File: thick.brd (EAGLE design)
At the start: 37 x 25 mm, 27 parts, among them J1 43045-0400, J4 F1003WR-S-06PT, Q1 SI2319DDS-T1-GE3, U1 ATTINY85-20SU

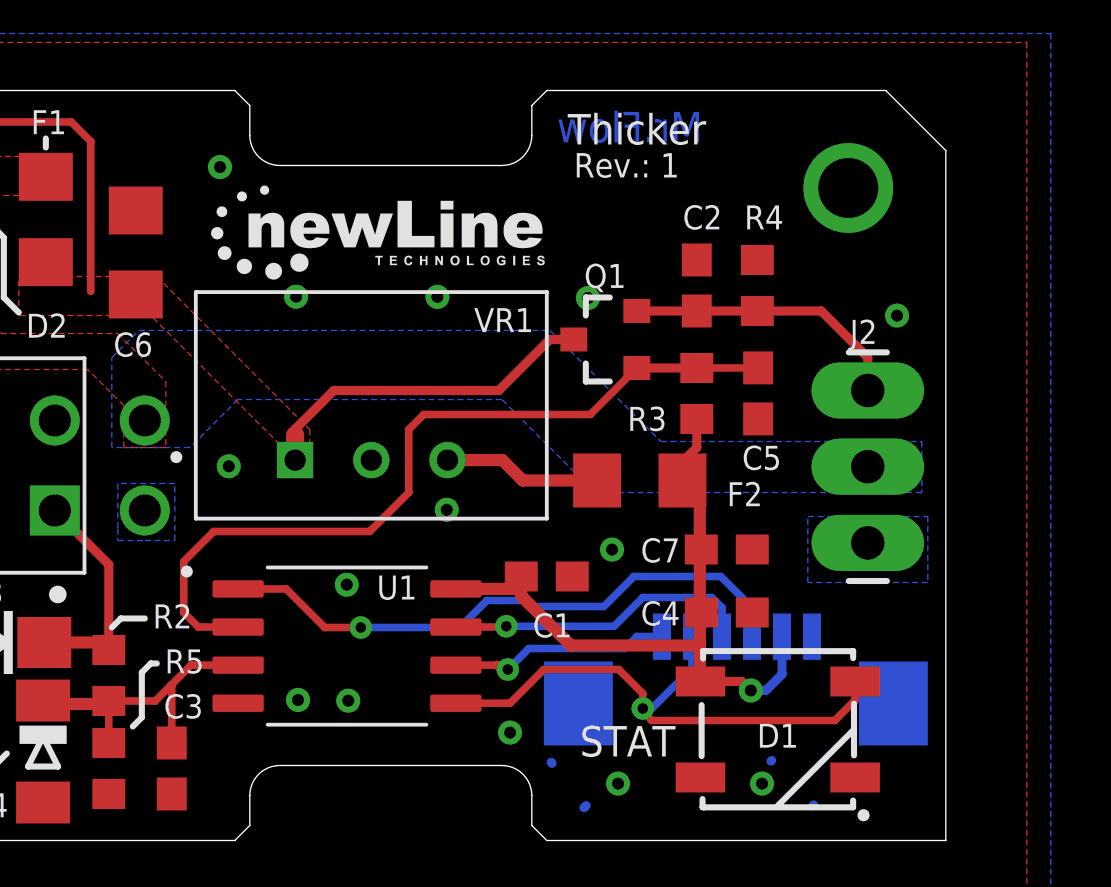
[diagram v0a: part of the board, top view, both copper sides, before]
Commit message: Javított végleges
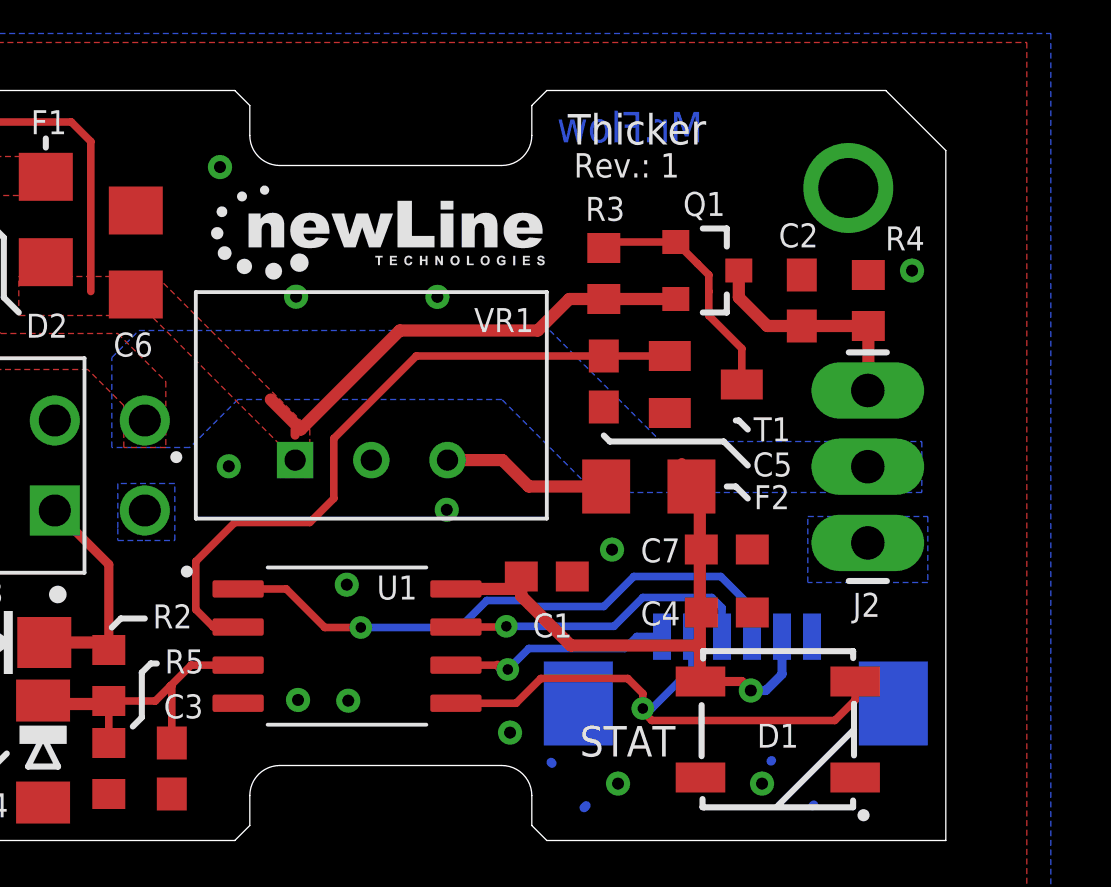
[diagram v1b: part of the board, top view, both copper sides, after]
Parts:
- added T1: (no value), transistor:SC59-BEC
- moved C5 5.16 mm to (25.6, 15.3)
- moved R3 5.06 mm to (25.6, 18.9)
- moved Q1 4.02 mm to (29.0, 19.0), turned to 270 degrees
- moved R4 3.73 mm to (34.4, 18.0)
- moved C2 3.54 mm to (32.2, 18.0)
- moved F2 0.36 mm to (27.1, 11.8)
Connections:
- removed net !IGN_EN: C5.1, Q1.1, R3.1, U1.2
- new net IGN_EN: C5.1, T1.B, U1.2
- new net N$1: Q1.1, R3.1, T1.C
- net 5V: no longer R3.2
- net GND: now also T1.E
- net IGNITION: now also Q1.3; no longer Q1.2
- net VDD: now also Q1.2, R3.2; no longer Q1.3
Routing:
- net !IGN_EN: track 26.8 -> 0.00 mm
- net IGN_EN: track 0.00 -> 23.1 mm
- net N$1: track 0.00 -> 8.14 mm
- net VDD: track 24.0 -> 28.2 mm
- net IGNITION: track 9.44 -> 7.77 mm
- net 5V: track 23.6 -> 22.0 mm
- net GND: vias 19 -> 18

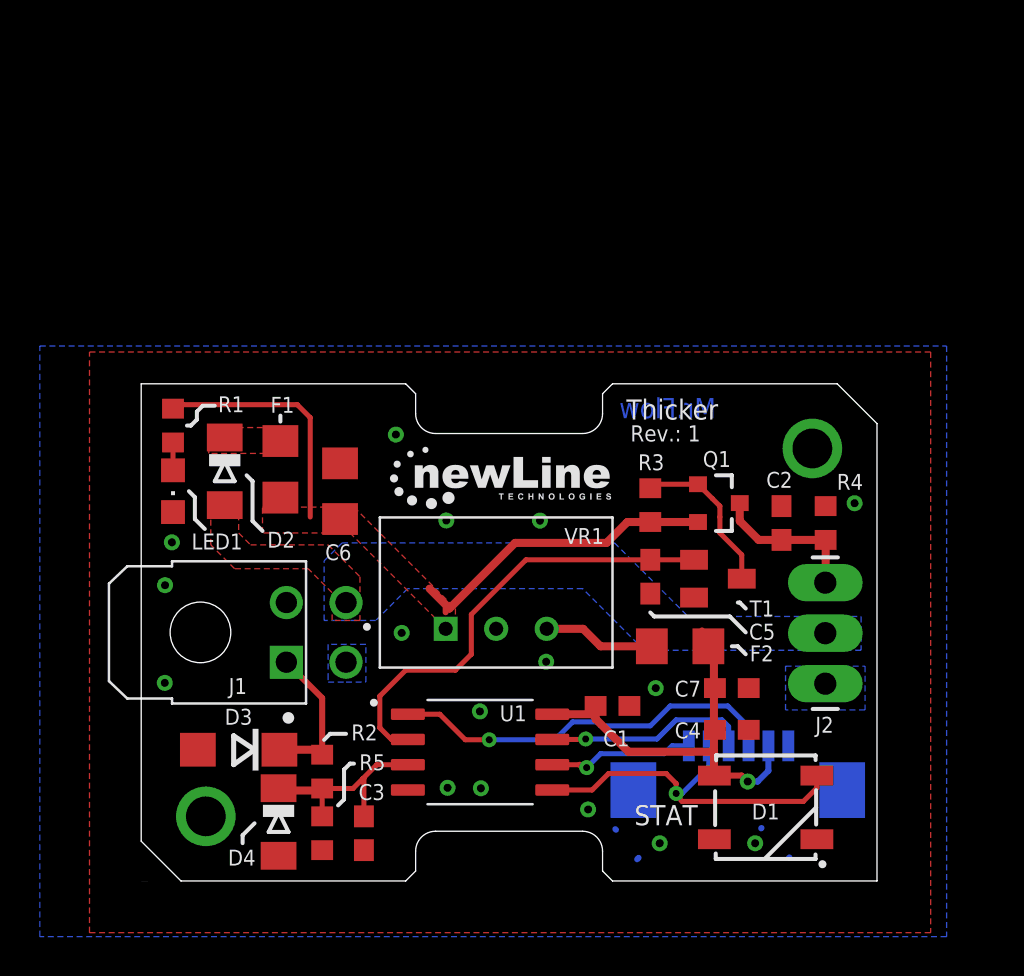
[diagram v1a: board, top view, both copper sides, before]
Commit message: rev 2
new pcb design with gerbers
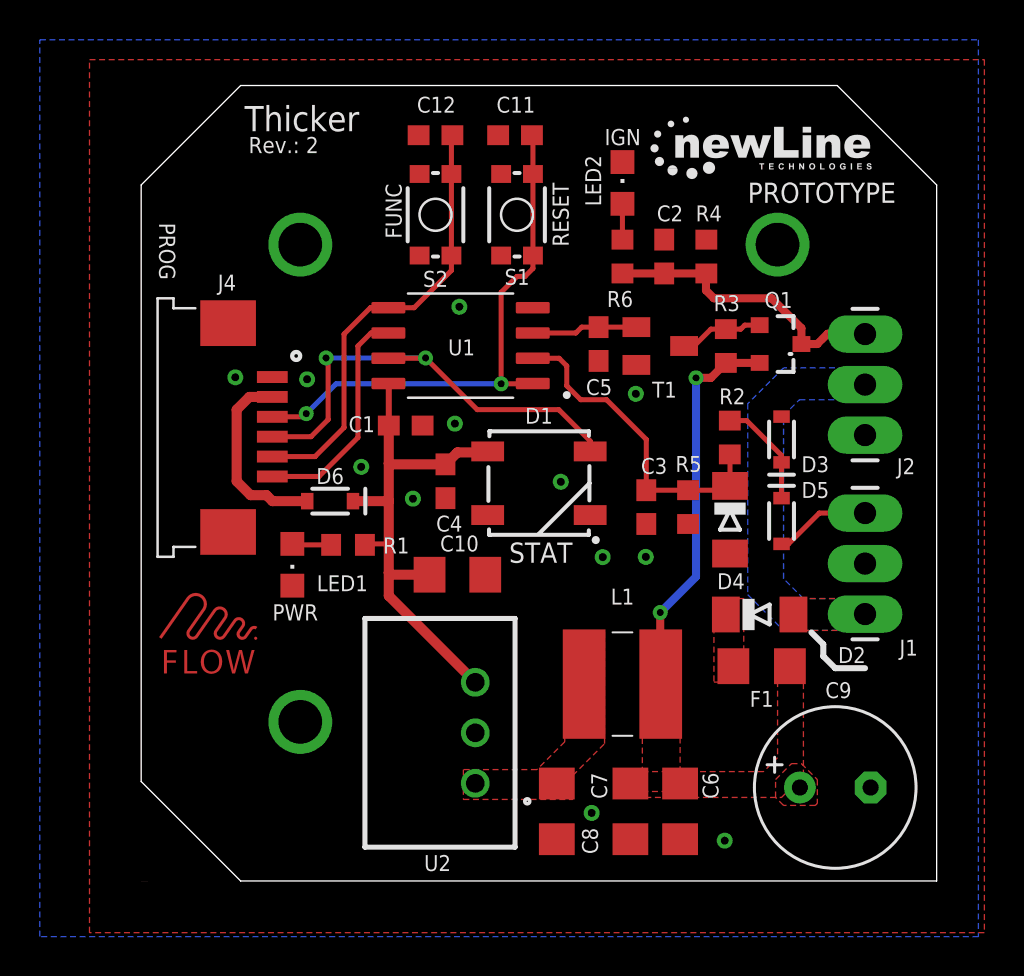
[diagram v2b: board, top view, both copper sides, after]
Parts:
- removed F2: (no value), adafruit:R1206
- removed VR1: VR05S05, TSR_1-24150:CONV_TSR_1-24150
- added C10, C8: 4.7uF, resistor:C1206
- added C11, C12: 0.1uF, resistor:C0603
- added C9: 100uF, resistor:E3,5-8
- added D5, D6: 0.5A/40V/420mV, SparkFun-DiscreteSemi:SOD-323
- added L1: TCK-047, TCK-047:TCK047
- added LED2: (no value), adafruit:CHIPLED_0805
- added R6: 10K, resistor:R0603
- added S1, S2: (no value), SparkFun-Switches:TACTILE_SWITCH_SMD_4.6X2.8MM
- added U$3: (no value), SparkFun-Aesthetics:ROHS_LOGO_0.18_IN
- added U$5: (no value), FloManEagle:MRFLOW_7_5MM
- added U2: TSR_0.5-2450, TSR_0.5-2450:TSR-0.5-2433
- C6: value 10uF -> 4.7uF
- C7: value 22uF -> 4.7uF; device resistor:C0603 -> resistor:C1206
- D3: value TVS -> tvs; device diode:DO214AC -> SparkFun-DiscreteSemi:SOD-323
- J1: value 43045-0400 -> (none); device 43045-0400:MOLEX_43045-0400 -> SparkFun-Connectors:1X03_LONGPADS
- moved J1 32.5 mm to (36.4, 18.5)
- moved U$1 32.3 mm to (25.0, 30.3)
- moved D3 31.4 mm to (32.2, 22.2), turned to 90 degrees
- moved J4 30.1 mm to (5.32, 22.8), flipped to the top, turned to 270 degrees
- moved D2 27.8 mm to (31.1, 13.4), turned to 0 degrees
- moved D4 27.3 mm to (29.6, 18.2)
- moved R2 26.5 mm to (29.6, 22.3)
- moved F1 26.1 mm to (31.2, 10.8), turned to 0 degrees
- moved U$2 25.1 mm to (20.0, 25.7)
- moved R5 24.6 mm to (27.5, 18.8)
- moved C6 23.5 mm to (27.1, 3.50), turned to 270 degrees
- moved C3 21.7 mm to (25.4, 18.8)
- moved U1 20.5 mm to (16.1, 26.9), turned to 180 degrees
- moved D1 19.9 mm to (20.0, 20.0)
- moved C4 19.1 mm to (15.3, 20.1), turned to 270 degrees
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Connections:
- new net N$2: C8.1, L1.2, U2.1
- new net N$5: D6.A, J4.2
- new net N$6: D3.C, D5.C, R2.1
- net !RESET: now also C11.1, S1.1, S1.2
- net 5V: now also C10.1, D6.C, R1.1, U2.3; no longer C7.1, F2.2, J4.2
- net AIN: now also U1.2; no longer U1.3
- net GND: now also C10.2, C11.2, C12.2, C8.2, C9.-, J1.2, LED2.C, S1.3, S1.4, S2.3, S2.4, U2.2; no longer J1.3, VR1.2
- net IGNITION: now also R6.1
- net IGN_EN: now also U1.3; no longer U1.2
- net MOSI: now also C12.1, S2.1, S2.2; no longer D1.4
- net N$4: now also LED2.A, R6.2; no longer F2.1, VR1.3
- net SCK: now also D1.4
- net SIGNAL: now also D5.A; no longer D3.C, R2.1
- net VCC: now also J1.3; no longer J1.4
- net VDD: now also C7.1, C9.+, L1.1; no longer R1.1, VR1.1
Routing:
- net IGN_EN: track 23.1 -> 5.33 mm
- net SCK: track 10.4 -> 23.7 mm, vias 1 -> 2
- net N$5: track 0.00 -> 9.62 mm
- net VDD: track 28.2 -> 19.7 mm, vias 0 -> 2
- net !RESET: track 19.9 -> 27.2 mm, vias 1 -> 2
- net IGNITION: track 7.77 -> 14.9 mm
- net AIN: track 10.4 -> 16.4 mm
- net N$6: track 0.00 -> 5.47 mm
- net 5V: track 22.0 -> 27.2 mm, vias 1 -> 0
- net MISO: track 7.39 -> 11.5 mm, vias 1 -> 0
- net N$1: track 8.14 -> 4.23 mm
- net N$4: track 5.65 -> 1.80 mm
- net MOSI: track 18.7 -> 22.5 mm, vias 1 -> 0
- net SIGNAL: track 7.65 -> 4.84 mm
- net N$3: track 1.40 -> 1.97 mm
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- added copper zone on layer 1, net N$2
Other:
- board size 37 x 25 mm -> 40 x 40 mm
- board text added: "2022.01.06."
- board text added: "FUNC"
- board text added: "INPUT"
- board text added: "Manufacturer: Szekely Florian ev. florian@mrflow.hu"
- board text added: "OUTPUT"
- board text added: "PROG"
- board text added: "PROTOTYPE"
- board text added: "PWR"
- board text added: "RESET"
- board text added: "Rev.: 2"
- board text added: "SGN"
- board text added: "VIN: 6.5-36VDC"
- board text removed: "2021.06.30."
- board text removed: "ISP"
- board text removed: "Mr.Flow"
- board text removed: "NewLine Kft. https://newline.hu/ Copyright (c) 2021"
- board text removed: "Rev.: 1"
- board text removed: "S/N:"
- board text removed: "VIN: 6.5-36VDC 2.5W"
